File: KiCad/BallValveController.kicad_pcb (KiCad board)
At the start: 2 copper layers, 55.6 x 43.2 mm, 62 parts, among them J1 Screw_Terminal_01x03, J2 Screw_Terminal_01x04, J3 Screw_Terminal_01x04, J4 Screw_Terminal_01x04, J5 Conn_01x01_Male, J6 Screw_Terminal_01x04, J7 Screw_Terminal_01x02, K1 G5V-2, Q1 Q_PMOS_GDS, Q2 2N2222A, U2 L7805, U3 XIAO-ESP32-C6, U4 TPS561201/08 or TPS563200

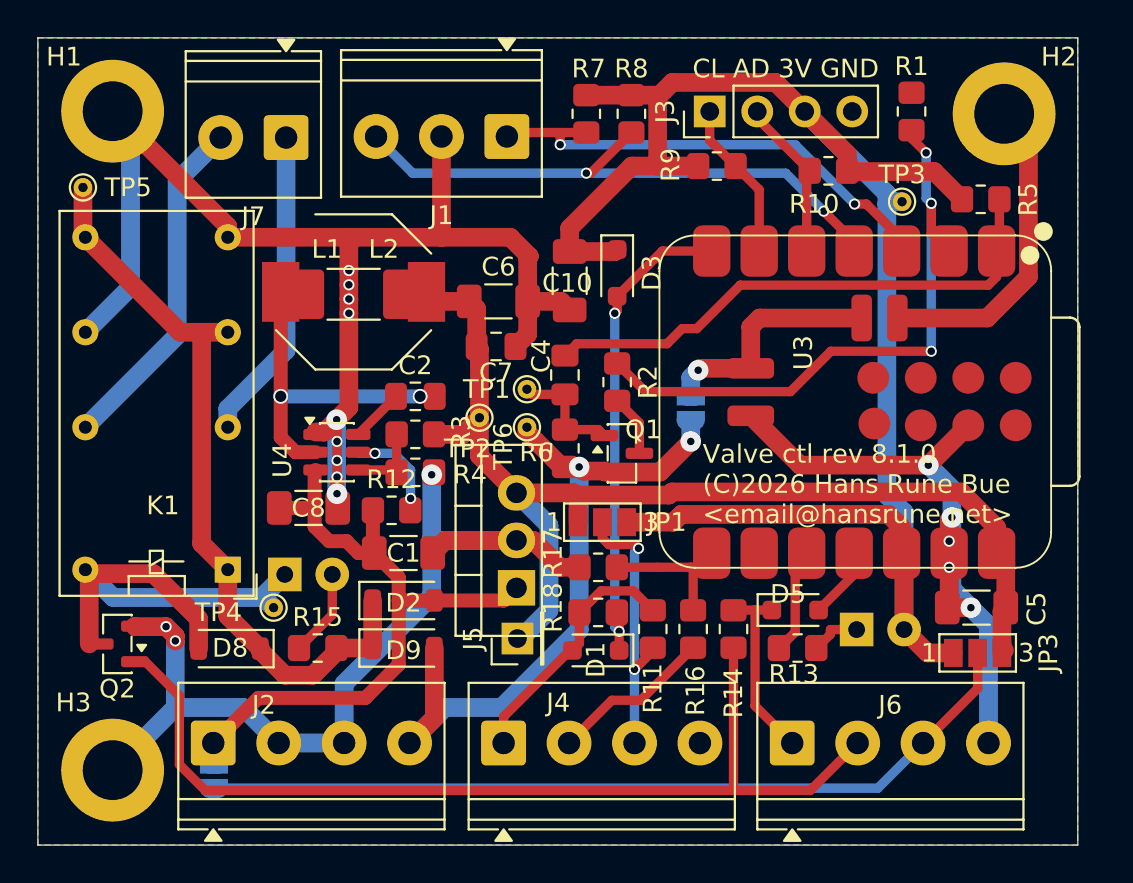
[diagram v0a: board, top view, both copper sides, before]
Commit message: ME3116 layout
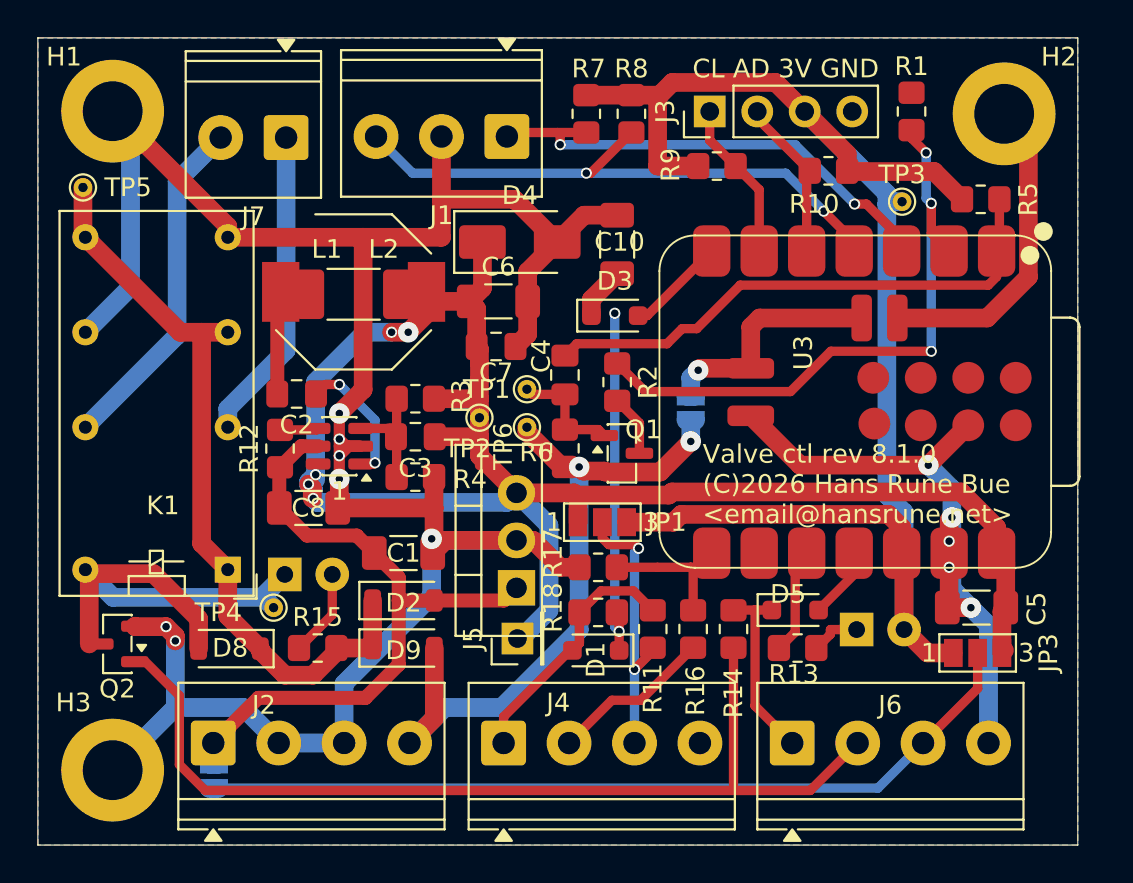
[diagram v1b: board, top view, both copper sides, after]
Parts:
- removed U4: TPS561201/08 or TPS563200, Package_TO_SOT_SMD:SOT-23-6
- added 1: ~, Package_TO_SOT_SMD:SOT-23-6, F.Cu at (152.0, 103.0)
- added C3: 470nF, Capacitor_SMD:C_0805_2012Metric_Pad1.18x1.45mm_HandSolder, F.Cu at (156.1, 102.5)
- added D4: SS34, Diode_SMD:D_SMA, F.Cu at (161.7, 92.1)
- moved R12 6.82 mm to (148.8, 103.1), turned to 90 degrees
- moved C2 6.35 mm to (149.7, 100.2), turned to 180 degrees
- moved C10 3.20 mm to (166.9, 92.2), turned to 90 degrees
- moved D3 2.29 mm to (166.8, 96.0), turned to 0 degrees
- moved R3 1.91 mm to (156.1, 100.5)
- moved R4 0.25 mm to (156.1, 104.6)
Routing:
- net +5V: track 61.2 -> 94.6 mm, vias 0 -> 5
- net /IND1: track 18.2 -> 5.54 mm, vias 2 -> 0
- net GND: track 175.6 -> 183.1 mm, vias 17 -> 12
- net +3V3: track 94.0 -> 86.9 mm
- net Net-(1-BS): track 2.87 -> 7.23 mm, vias 0 -> 2
- net Net-(1-EN): track 5.36 -> 2.07 mm, vias 2 -> 0
- net Net-(1-FB): track 4.14 -> 6.76 mm
- net Net-(D1-K): track 26.2 -> 24.6 mm
